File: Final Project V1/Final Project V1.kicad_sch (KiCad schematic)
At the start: 30 parts, among them J1 39299043, Q1 SS8050-G, Q2 SS8050-G, SW1 SW_Push, SW2 SW_Push, U1 AP2112K-3.3, U2 ESP32-S3-WROOM-1, U3 BQ21040DBVR

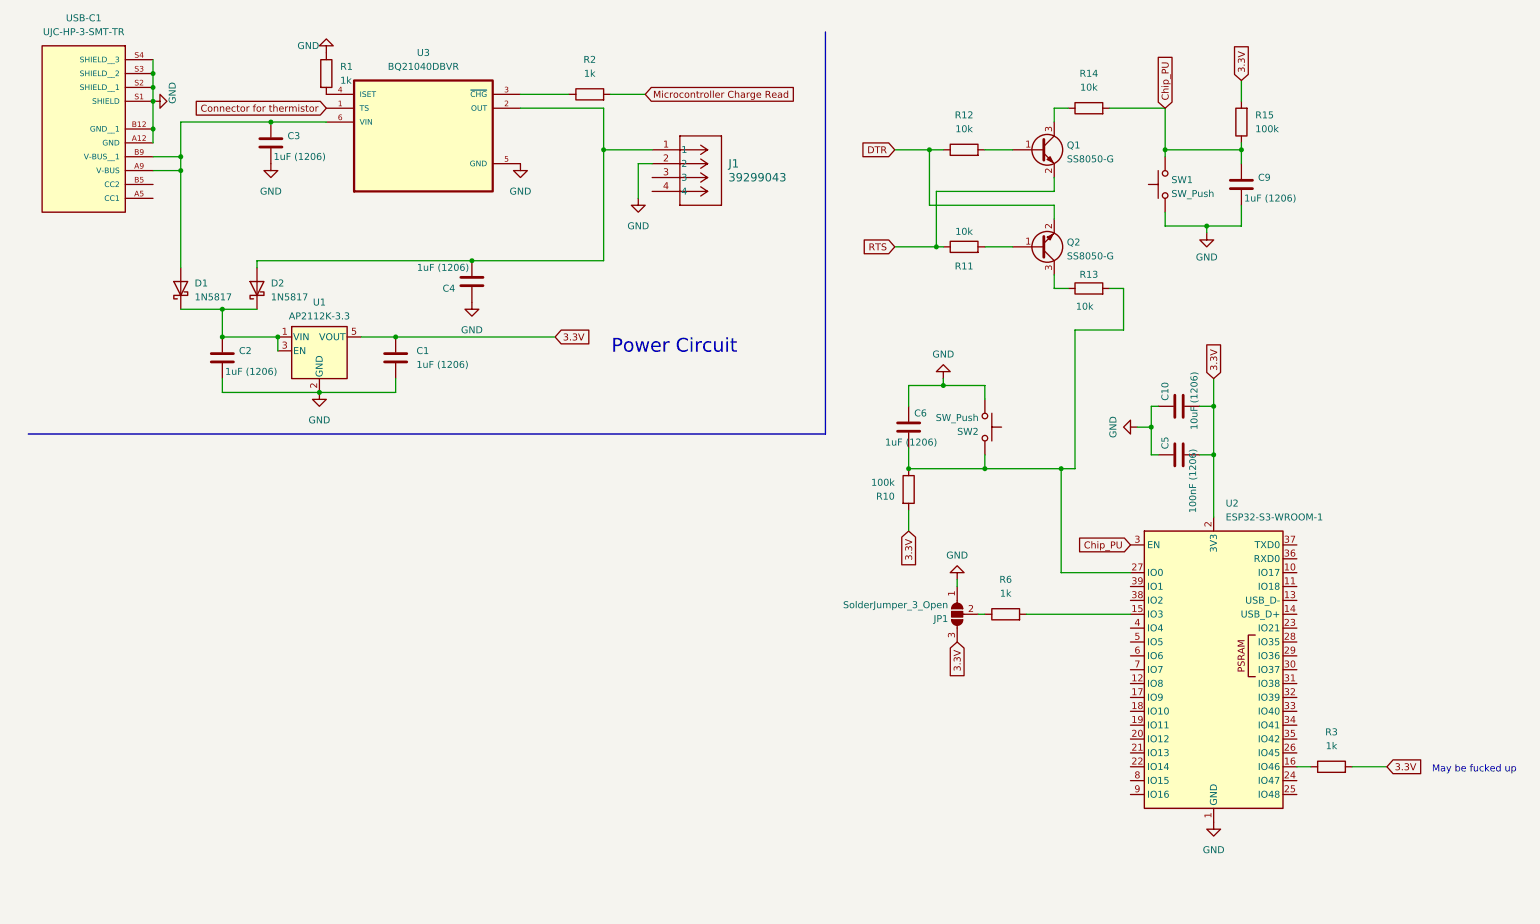
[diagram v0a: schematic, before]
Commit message: Finish V1 Board
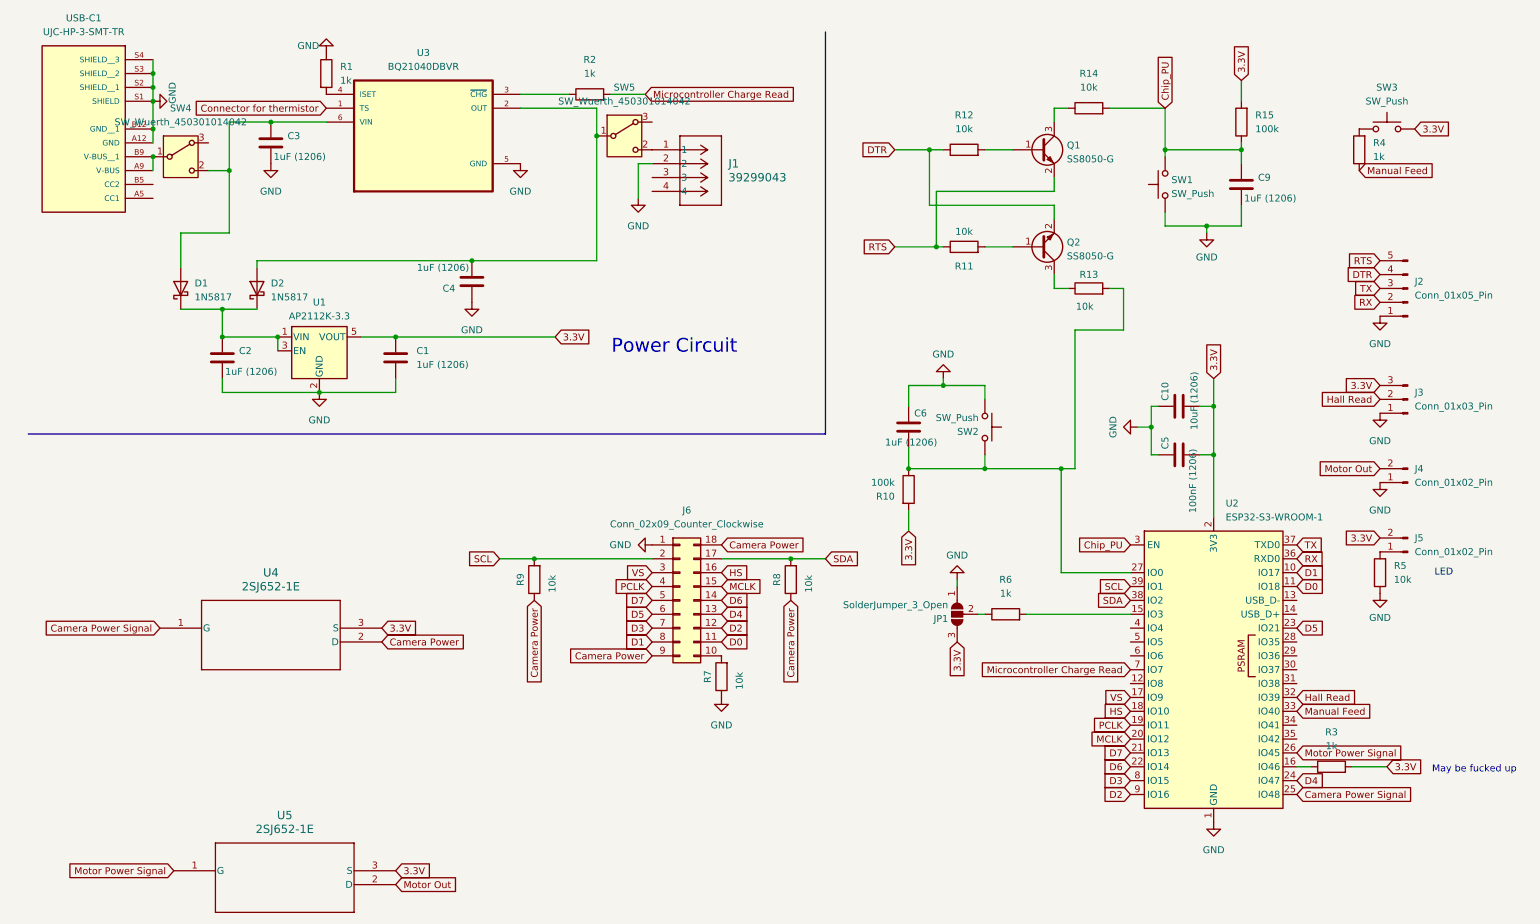
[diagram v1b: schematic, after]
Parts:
- added J2: Conn_01x05_Pin, Connector_PinSocket_2.54mm:PinSocket_1x05_P2.54mm_Vertical, symbol Connector:Conn_01x05_Pin
- added J3: Conn_01x03_Pin, Connector_PinSocket_2.54mm:PinSocket_1x03_P2.54mm_Vertical, symbol Connector:Conn_01x03_Pin
- added J4, J5: Conn_01x02_Pin, Connector_PinSocket_2.54mm:PinSocket_1x02_P2.54mm_Vertical, symbol Connector:Conn_01x02_Pin
- added J6: Conn_02x09_Counter_Clockwise, Connector_PinSocket_2.54mm:PinSocket_2x09_P2.54mm_Vertical, symbol Connector_Generic:Conn_02x09_Counter_Clockwise
- added R4: 1k, Resistor_SMD:R_0805_2012Metric_Pad1.20x1.40mm_HandSolder, symbol Device:R
- added R5, R7, R8, R9: 10k, Resistor_SMD:R_0805_2012Metric_Pad1.20x1.40mm_HandSolder, symbol Device:R
- added SW3: SW_Push, Button_Switch_SMD:SW_SPST_B3S-1000, symbol Switch:SW_Push
- added SW4, SW5: SW_Wuerth_450301014042, Button_Switch_THT:SW_Slide-03_Wuerth-WS-SLTV_10x2.5x6.4_P2.54mm, symbol Switch:SW_Wuerth_450301014042
- added U4, U5: 2SJ652-1E, TO-220F-3SG_15P87X10P16_ONS, symbol 2SJ652-1E:2SJ652-1E
- R1, R10, R11, R12, R13, R14, R15, R2, R3, R6: footprint Resistor_SMD:R_1206_3216Metric_Pad1.30x1.75mm_HandSolder -> Resistor_SMD:R_0805_2012Metric_Pad1.20x1.40mm_HandSolder
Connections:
- net 3.3V: now also J3.3 (Pin_3), J5.2 (Pin_2), SW3.2, U4.3 (S), U5.3 (S)
- net DTR: now also J2.4 (Pin_4)
- net GND: now also J2.1 (Pin_1), J3.1 (Pin_1), J4.1 (Pin_1), J6.1 (Pin_1), R5.1, R7.1
- net Microcontroller Charge Read: now also U2.7 (IO7)
- net RTS: now also J2.5 (Pin_5)
- net at C3.1, D1.2 (A), U3.6 (VIN): now also SW4.2 (C); no longer USB-C1.A9 (V-BUS), USB-C1.B9 (V-BUS__1)
- net at C4.2, D2.2 (A), U3.2 (OUT): now also SW5.1 (B); no longer J1.1
- net D1: now reaches U2.10 (IO17)
- net D1: now also J6.8 (Pin_8)
- net D0: now reaches U2.11 (IO18)
- net D0: now also J6.11 (Pin_11)
- net VS: now reaches U2.17 (IO9)
- net VS: now also J6.3 (Pin_3)
- net HS: now reaches U2.18 (IO10)
- net HS: now also J6.16 (Pin_16)
- net PCLK: now reaches U2.19 (IO11)
- net PCLK: now also J6.4 (Pin_4)
- net MCLK: now reaches U2.20 (IO12)
- net MCLK: now also J6.15 (Pin_15)
- net D7: now reaches U2.21 (IO13)
- net D7: now also J6.5 (Pin_5)
- net D6: now reaches U2.22 (IO14)
- net D6: now also J6.14 (Pin_14)
- net D5: now reaches U2.23 (IO21)
- net D5: now also J6.6 (Pin_6)
- net D4: now reaches U2.24 (IO47)
- net D4: now also J6.13 (Pin_13)
- net Camera Power Signal: now reaches U2.25 (IO48)
- net Camera Power Signal: now also U4.1 (G)
- net Motor Power Signal: now reaches U2.26 (IO45)
- net Motor Power Signal: now also U5.1 (G)
- net Hall Read: now reaches U2.32 (IO39)
- net Hall Read: now also J3.2 (Pin_2)
- net Manual Feed: now reaches U2.33 (IO40)
- net Manual Feed: now also R4.1
- net RX: now reaches U2.36 (RXD0)
- net RX: now also J2.2 (Pin_2)
- net TX: now reaches U2.37 (TXD0)
- net TX: now also J2.3 (Pin_3)
- net SDA: now reaches U2.38 (IO2)
- net SDA: now also J6.17 (Pin_17), R8.2
- net SCL: now reaches U2.39 (IO1)
- net SCL: now also J6.2 (Pin_2), R9.2
- net D3: now reaches U2.8 (IO15)
- net D3: now also J6.7 (Pin_7)
- net D2: now reaches U2.9 (IO16)
- net D2: now also J6.12 (Pin_12)
- new net: J1.1, SW5.2 (C)
- new net: J5.1 (Pin_1), R5.2
- new net: R4.2, SW3.1
- new net: J6.10 (Pin_10), R7.2
- new net: SW4.1 (B), USB-C1.A9 (V-BUS), USB-C1.B9 (V-BUS__1)
- new net Camera Power: J6.18 (Pin_18), J6.9 (Pin_9), R8.1, R9.1, U4.2 (D)
- new net Motor Out: J4.2 (Pin_2), U5.2 (D)
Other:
- note added: "LED"
